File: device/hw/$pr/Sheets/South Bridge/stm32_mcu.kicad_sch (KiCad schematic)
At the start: 1 part, among them U5 STM32F411CEU6

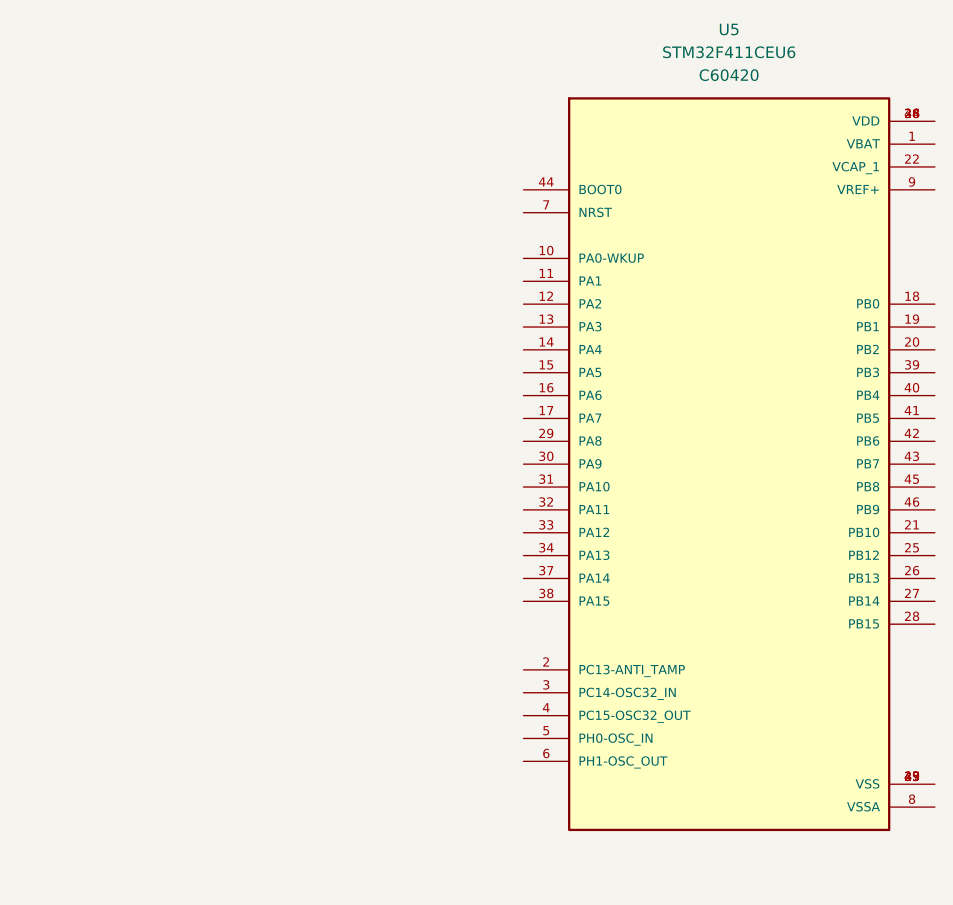
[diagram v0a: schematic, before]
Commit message: *
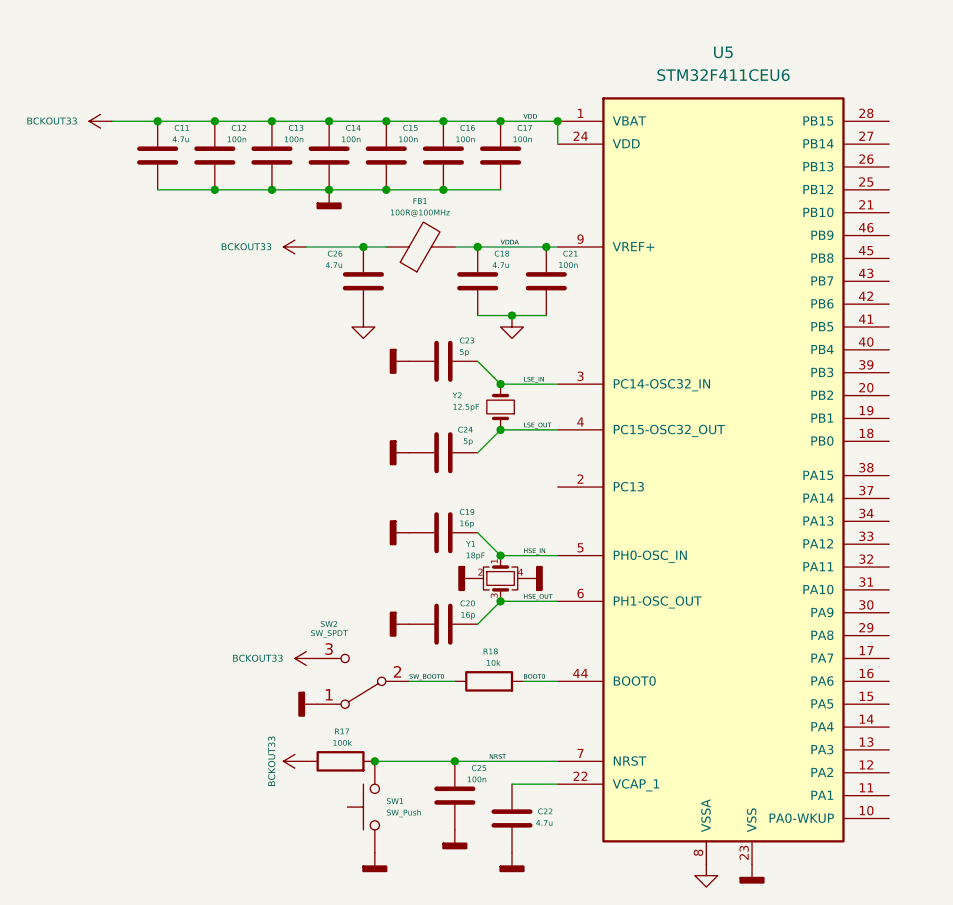
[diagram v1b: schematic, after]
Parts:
- added C11, C18, C22, C26: 4.7u, symbol Device:C
- added C12, C13, C14, C15, C16, C17, C21, C25: 100n, symbol Device:C
- added C19, C20: 16p, symbol Device:C
- added C23, C24: 5p, symbol Device:C
- added FB1: 100R@100MHz, Inductor_SMD:L_0805_2012Metric, symbol Device:FerriteBead
- added R17: 100k, symbol Device:R
- added R18: 10k, symbol Device:R
- added SW1: SW_Push, symbol Switch:SW_Push
- added SW2: SW_SPDT, symbol Switch:SW_SPDT
- added Y1: 18pF, Crystal:Crystal_SMD_3225-4Pin_3.2x2.5mm, symbol Device:Crystal_GND24_Small
- added Y2: 12.5pF, Crystal:Crystal_SMD_3215-2Pin_3.2x1.5mm, symbol Device:Crystal_Small
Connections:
- net BCKOUT33: now reaches U5.1 (VBAT)
- net BCKOUT33: now also U5.24 (VDD), U5.36 (VDD), U5.48 (VDD), C11.2, C12.2, C13.2, C14.2, C15.2, C16.2, C17.2, C26.2, FB1.1, R17.1, SW2.3 (C)
- net at U5.22 (VCAP_1): now also C22.2
- net GNDD: now reaches U5.23 (VSS), U5.35 (VSS), U5.47 (VSS), U5.49 (VSS)
- net GNDD: now also C11.1, C12.1, C13.1, C14.1, C15.1, C16.1, C17.1, C19.2, C20.1, C22.1, C23.2, C24.1, C25.1, SW1.1, SW2.1 (A), Y1.2, Y1.4
- net LSE_IN: now reaches U5.3 (PC14-OSC32_IN)
- net LSE_IN: now also C23.1, Y2.2
- net LSE_OUT: now reaches U5.4 (PC15-OSC32_OUT)
- net LSE_OUT: now also C24.2, Y2.1
- net BOOT0: now reaches U5.44 (BOOT0)
- net BOOT0: now also R18.2
- net HSE_IN: now reaches U5.5 (PH0-OSC_IN)
- net HSE_IN: now also C19.1, Y1.1
- net HSE_OUT: now reaches U5.6 (PH1-OSC_OUT)
- net HSE_OUT: now also C20.2, Y1.3
- net NRST: now reaches U5.7 (NRST)
- net NRST: now also C25.2, R17.2, SW1.2
- net GNDA: now reaches U5.8 (VSSA)
- net GNDA: now also C18.1, C21.1, C26.1
- net VDDA: now reaches U5.9 (VREF+)
- net VDDA: now also C18.2, C21.2, FB1.2
- new net SW_BOOT0: R18.1, SW2.2 (B)
